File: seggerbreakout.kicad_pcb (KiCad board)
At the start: 2 copper layers, 29.5 x 28 mm, 3 parts, among them P1 SWD, P2 JTAG, P3 JTAG

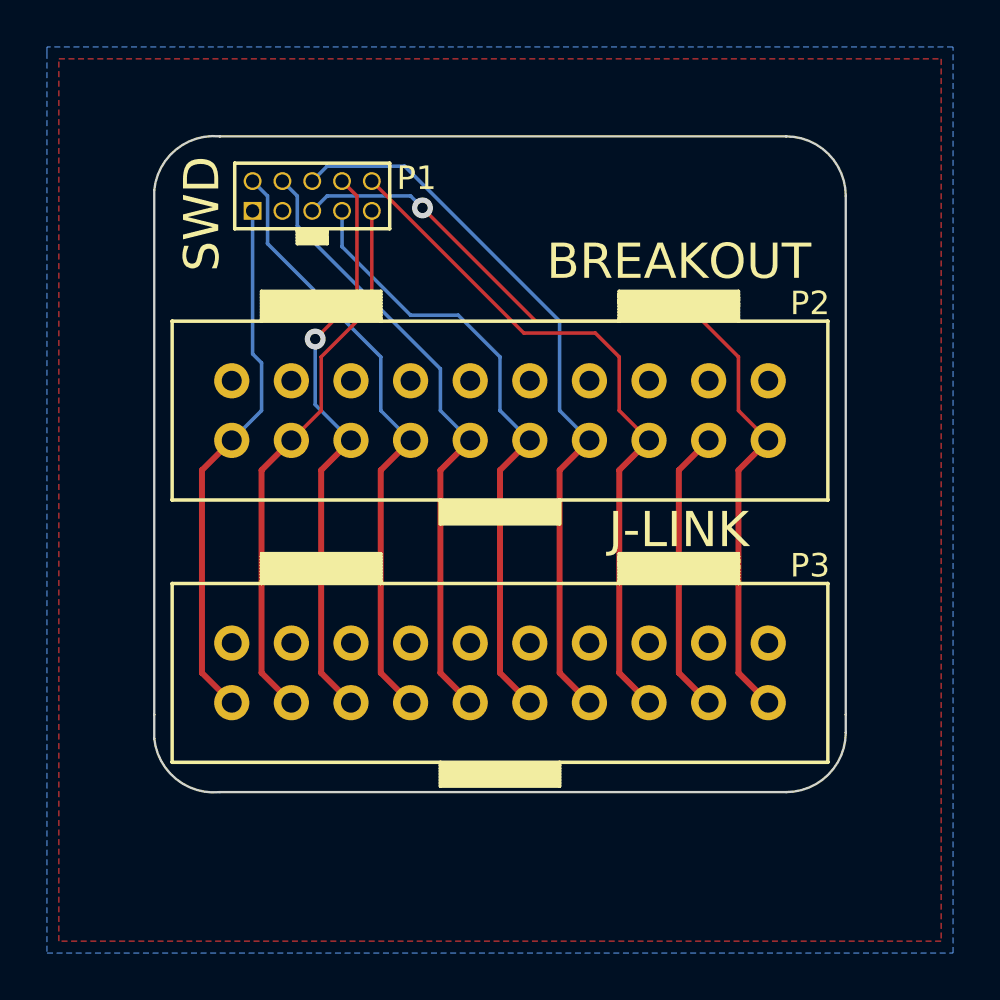
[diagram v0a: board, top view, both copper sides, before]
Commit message: Sent to fab
Vendor: OSHPark, LLC
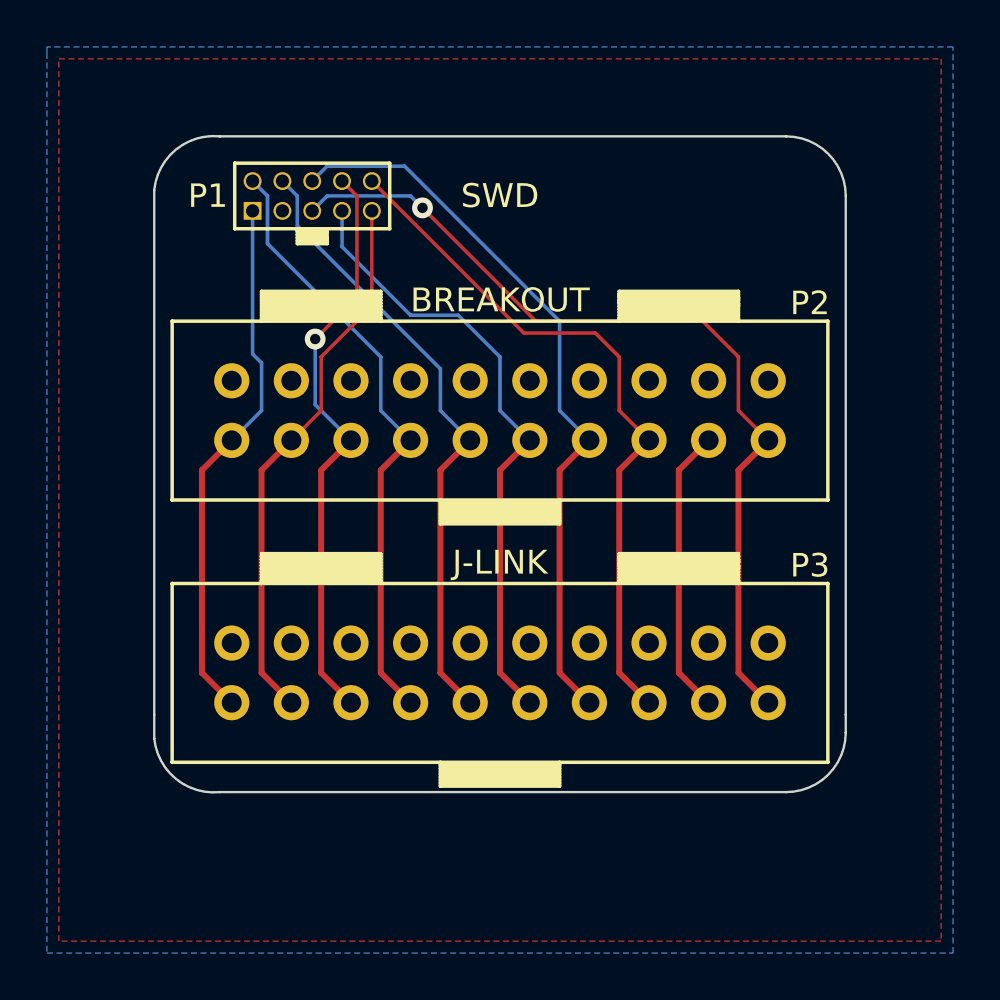
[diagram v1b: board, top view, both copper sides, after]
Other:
- board text added: "J-LINK Breakout+SWD 2014-08-31 open.konspyre.org/jswd"
- board text removed: "J-LINK Breakout+SWD 2014-08-18 open.konspyre.org/jswd"
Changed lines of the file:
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@@
     (area 179.07 114.554 217.678001 153.162001)
     (thickness 1.6)
-    (drawings 74)
+    (drawings 71)
     (tracks 79)
     (zones 0)
@@
   (page A3)
   (layers
-    (15 F.Cu signal)
-    (0 B.Cu signal)
+    (15 F.Cu signal hide)
+    (0 B.Cu signal hide)
     (16 B.Adhes user)
     (17 F.Adhes user)
@@
   (module JTAG_SMALL (layer F.Cu)
     (at 189.738 120.904 180)
-    (fp_text reference P1 (at -5.08 0.762 180) (layer F.SilkS)
+    (fp_text reference P1 (at 3.81 0 180) (layer F.SilkS)
       (effects (font (size 1 1) (thickness 0.15)))
     )
@@
     )
   )
+  (gr_line (start 196.85 126.238) (end 196.85 125.984) (angle 90) (layer B.SilkS) (width 0.2))
+  (gr_line (start 192.024 126.746) (end 192.024 127.762) (angle 90) (layer B.SilkS) (width 0.2))
+  (gr_line (start 189.484 127.508) (end 189.484 127.762) (angle 90) (layer B.SilkS) (width 0.2))
   (gr_line (start 188.214 133.35) (end 188.214 133.604) (angle 90) (layer B.SilkS) (width 0.2))
   (gr_line (start 207.264 132.588) (end 207.264 133.35) (angle 90) (layer B.SilkS) (width 0.2))
@@
   (gr_line (start 186.944 133.35) (end 189.484 133.35) (angle 90) (layer B.SilkS) (width 0.2))
   (gr_line (start 186.944 132.588) (end 186.944 133.35) (angle 90) (layer B.SilkS) (width 0.2))
-  (gr_text "J-LINK Breakout+SWD\n2014-08-18\nopen.konspyre.org/jswd" (at 202.438 134.62) (layer B.SilkS)
+  (gr_text "J-LINK Breakout+SWD\n2014-08-31\nopen.konspyre.org/jswd" (at 202.438 134.62) (layer B.SilkS)
     (effects (font (size 1.0668 1.0668) (thickness 0.2667)) (justify mirror))
   )
-  (gr_text BREAKOUT (at 205.994 123.698) (layer F.SilkS)
-    (effects (font (size 1.5 1.5) (thickness 0.3)))
-  )
-  (gr_text J-LINK (at 205.994 135.128) (layer F.SilkS)
-    (effects (font (size 1.5 1.5) (thickness 0.3)))
-  )
-  (gr_text SWD (at 185.674 121.666 90) (layer F.SilkS)
-    (effects (font (size 1.5 1.5) (thickness 0.3)))
+  (gr_text BREAKOUT (at 198.374 125.349) (layer F.SilkS)
+    (effects (font (size 1.016 1.016) (thickness 0.254)))
+  )
+  (gr_text J-LINK (at 198.374 136.525) (layer F.SilkS)
+    (effects (font (size 1.016 1.016) (thickness 0.254)))
+  )
+  (gr_text SWD (at 198.374 120.904) (layer F.SilkS)
+    (effects (font (size 1.016 1.016) (thickness 0.254)))
   )
   (gr_text GND (at 188.214 134.874) (layer B.SilkS)
@@
   )
   (gr_line (start 199.39 125.476) (end 199.39 124.968) (angle 90) (layer B.SilkS) (width 0.2))
-  (gr_line (start 201.676 125.476) (end 201.676 124.968) (angle 90) (layer B.SilkS) (width 0.2))
-  (gr_line (start 196.85 126.238) (end 196.85 125.73) (angle 90) (layer B.SilkS) (width 0.2))
-  (gr_line (start 192.024 127) (end 192.024 126.492) (angle 90) (layer B.SilkS) (width 0.2))
   (gr_line (start 186.944 127.508) (end 186.944 127.762) (angle 90) (layer B.SilkS) (width 0.2))
   (gr_line (start 209.804 127.508) (end 209.804 127.762) (angle 90) (layer B.SilkS) (width 0.2))
@@
   (gr_line (start 197.104 127.508) (end 197.104 127.762) (angle 90) (layer B.SilkS) (width 0.2))
   (gr_line (start 194.564 127.508) (end 194.564 127.762) (angle 90) (layer B.SilkS) (width 0.2))
-  (gr_line (start 192.024 127.508) (end 192.024 127.762) (angle 90) (layer B.SilkS) (width 0.2))
-  (gr_line (start 189.484 127.254) (end 189.484 127.762) (angle 90) (layer B.SilkS) (width 0.2))
-  (gr_line (start 192.024 127) (end 192.024 127.508) (angle 90) (layer B.SilkS) (width 0.2))
   (gr_line (start 194.564 125.476) (end 194.564 127.508) (angle 90) (layer B.SilkS) (width 0.2))
   (gr_line (start 197.104 126.492) (end 197.104 127.508) (angle 90) (layer B.SilkS) (width 0.2))
@@
   (gr_line (start 209.042 126.492) (end 209.804 127.254) (angle 90) (layer B.SilkS) (width 0.2))
   (gr_line (start 186.944 124.46) (end 186.944 127.508) (angle 90) (layer B.SilkS) (width 0.2))
-  (gr_text "5V\nDBGRQ\nRESET\nTDO\nRTCK\nTCK\nTMS\nTDI\nnTRST\nVTref" (at 187.452 121.92 90) (layer B.SilkS)
+  (gr_text "5V\nDBGRQ\nRESET\nTDO\nRTCK\nTCK\nTMS\nTDI\nnTRST\nVTref" (at 187.452 122.174 90) (layer B.SilkS)
     (effects (font (size 1.524 1.016) (thickness 0.254)) (justify left mirror))
   )
